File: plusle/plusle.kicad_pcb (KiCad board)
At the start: 2 copper layers, 72.9 x 31 mm, 6 parts, among them J1 Battery, J2 MotorA, J3 MotorB, U1 ESP32-DEVKIT-V1, U2 ROB-14450

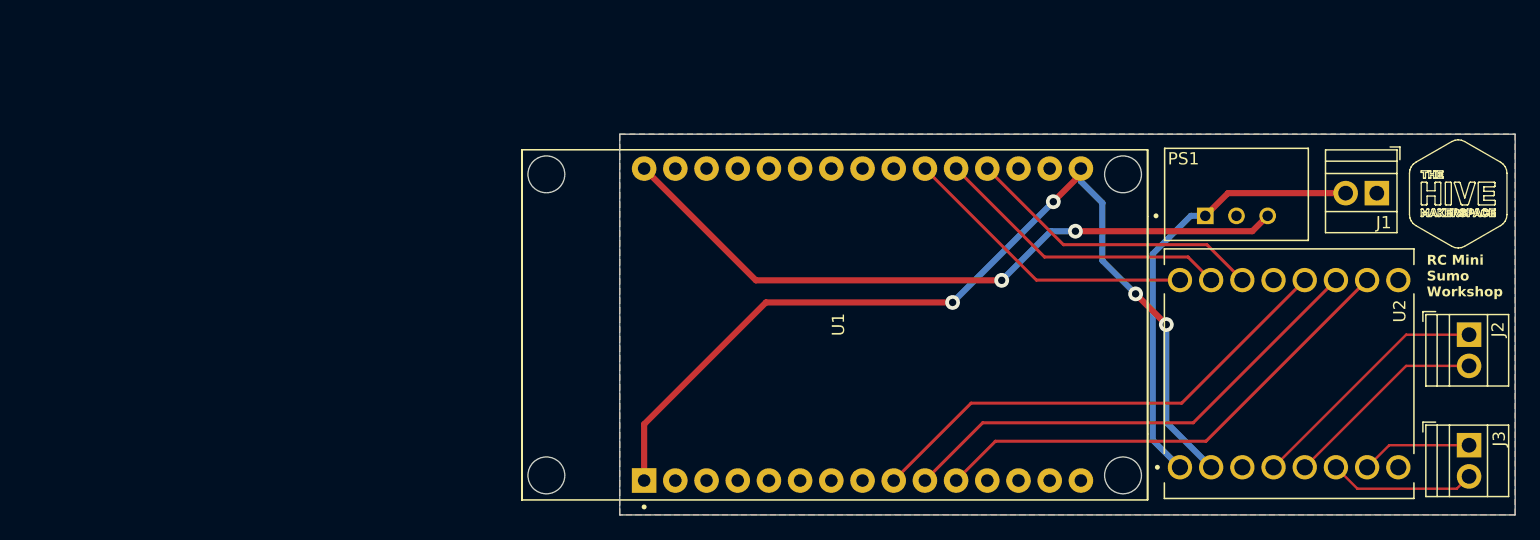
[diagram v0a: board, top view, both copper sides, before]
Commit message: NewIteration
new compact board for personal plusle project, non-hive
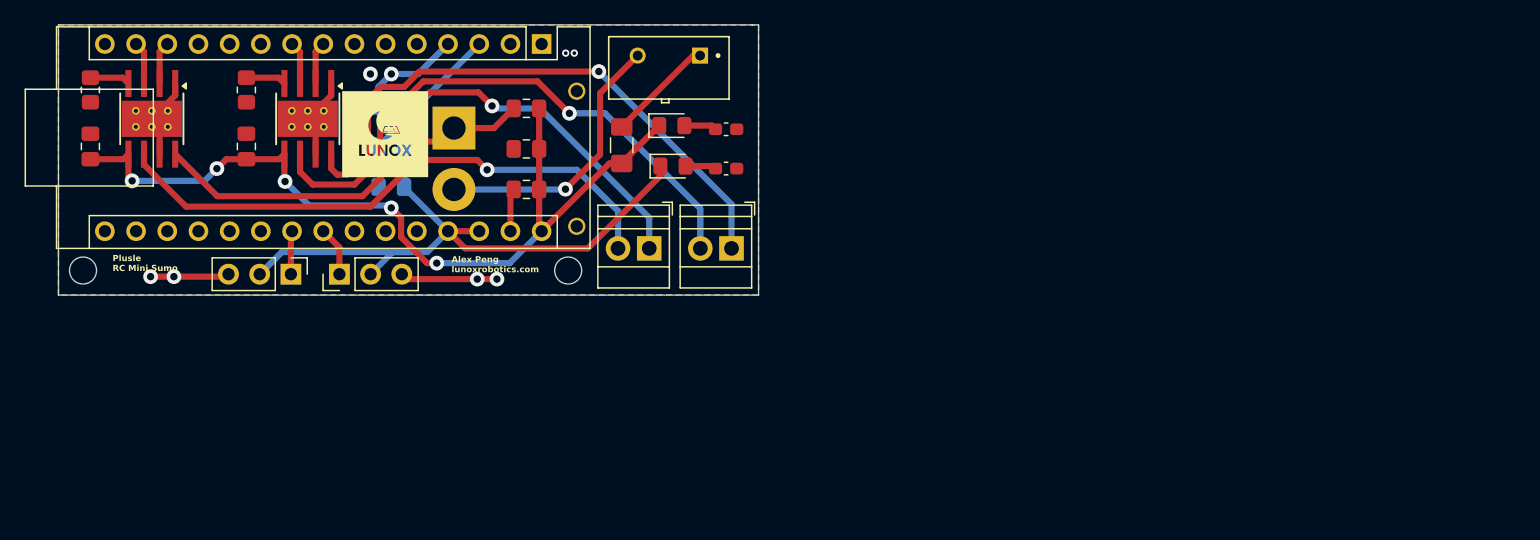
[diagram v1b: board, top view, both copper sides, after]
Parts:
- removed PS1: TSR_1-2450, TSR_1-2433:CONV_TSR_1-2433
- removed U1: ESP32-DEVKIT-V1, Library:MODULE_ESP32_DEVKIT_V1
- removed U2: ROB-14450, Library:MODULE_ROB-14450
- added A1: Arduino_Nano_v3.x, Module:Arduino_Nano, F.Cu at (65.1, 28.2)
- added C1: 0.1uf, Capacitor_SMD:C_0805_2012Metric_Pad1.18x1.45mm_HandSolder, F.Cu at (63.9, 33.4)
- added C2: 0.1uf, Capacitor_SMD:C_0805_2012Metric_Pad1.18x1.45mm_HandSolder, F.Cu at (63.9, 36.7)
- added C3: 0.1uf, Capacitor_SMD:C_0805_2012Metric_Pad1.18x1.45mm_HandSolder, F.Cu at (63.9, 40.0)
- added C4: 0.1uf, Capacitor_SMD:C_0805_2012Metric_Pad1.18x1.45mm_HandSolder, B.Cu at (52.9, 39.8)
- added C5: 0.1uf, Capacitor_SMD:C_0805_2012Metric_Pad1.18x1.45mm_HandSolder, B.Cu at (52.9, 36.5)
- added C6: 0.1uf, Capacitor_SMD:C_0805_2012Metric_Pad1.18x1.45mm_HandSolder, B.Cu at (52.9, 33.2)
- added C7: 0.1uf, Capacitor_SMD:C_0805_2012Metric_Pad1.18x1.45mm_HandSolder, F.Cu at (28.4, 36.5)
- added C8: 0.1uf, Capacitor_SMD:C_0805_2012Metric_Pad1.18x1.45mm_HandSolder, F.Cu at (41.1, 36.5)
- added D1: GREEN, Capacitor_SMD:C_0603_1608Metric_Pad1.08x0.95mm_HandSolder, F.Cu at (80.2, 35.1)
- added D2: GREEN, Capacitor_SMD:C_0603_1608Metric_Pad1.08x0.95mm_HandSolder, F.Cu at (80.2, 38.3)
- added F1: 15A, Fuse:Fuse_1206_3216Metric_Pad1.42x1.75mm_HandSolder, F.Cu at (71.7, 36.4)
- added G***: LOGO, LOGO, F.Cu at (52.4, 35.5)
- added H1: MountingHole, MountingHole:MountingHole_2.2mm_M2_ISO7380, F.Cu at (27.8, 46.6)
- added H2: MountingHole, MountingHole:MountingHole_2.2mm_M2_ISO7380, F.Cu at (67.3, 46.6)
- added J4: Receiver Connection1, Connector_PinHeader_2.54mm:PinHeader_1x03_P2.54mm_Vertical, F.Cu at (44.7, 46.9)
- added J5: Battery, Connector_AMASS:AMASS_XT30PW-M_1x02_P2.50mm_Horizontal, B.Cu at (58.0, 35.0)
- added R1: 15k, Resistor_SMD:R_0805_2012Metric_Pad1.20x1.40mm_HandSolder, F.Cu at (28.4, 31.9)
- added R2: 15k, Resistor_SMD:R_0805_2012Metric_Pad1.20x1.40mm_HandSolder, F.Cu at (41.1, 31.9)
- added R3: 600, Diode_SMD:D_0805_2012Metric_Pad1.15x1.40mm_HandSolder, F.Cu at (75.7, 34.8)
- added R4: 600, Diode_SMD:D_0805_2012Metric_Pad1.15x1.40mm_HandSolder, F.Cu at (75.8, 38.1)
- added SW1: SW_SPST, Button_Switch_THT:SW_AS11CP, F.Cu at (75.5, 30.1)
- added U3: DRV8871DDA, Package_SO:Texas_HTSOP-8-1EP_3.9x4.9mm_P1.27mm_EP2.95x4.9mm_Mask2.4x3.1mm_ThermalVias, F.Cu at (33.4, 34.2)
- added U4: DRV8871DDA, Package_SO:Texas_HTSOP-8-1EP_3.9x4.9mm_P1.27mm_EP2.95x4.9mm_Mask2.4x3.1mm_ThermalVias, F.Cu at (46.1, 34.2)
- J1: value Battery -> Receiver Connection2; footprint TerminalBlock:TerminalBlock_Xinya_XY308-2.54-2P_1x02_P2.54mm_Horizontal -> Connector_PinHeader_2.54mm:PinHeader_1x03_P2.54mm_Vertical
- moved J1 84.7 mm to (48.7, 46.9), turned to 90 degrees
- moved J2 67.1 mm to (73.9, 44.8), turned to 180 degrees
- moved J3 62.2 mm to (80.6, 44.8), turned to 180 degrees
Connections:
- J1 pad 1: GND -> RCSignalB
- J1 pad 2: +12V -> Arduino5V
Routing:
- net +3.3V: track 77.7 -> 0.00 mm, vias 4 -> 0
- net ArduinoVIN: track 0.00 -> 70.0 mm, vias 0 -> 5
- net Arduino5V: track 0.00 -> 67.5 mm
- net +5V: track 56.7 -> 0.00 mm, vias 2 -> 0
- net GND: track 0.00 -> 56.0 mm, vias 0 -> 11
- net PWMB: track 40.2 -> 0.00 mm
- net Net-(J3-Pin_1): track 9.04 -> 48.1 mm, vias 0 -> 1
- net BIn2: track 40.2 -> 3.47 mm
- net BIn1: track 40.2 -> 3.48 mm
- net Net-(J3-Pin_2): track 12.0 -> 48.1 mm, vias 0 -> 1
- net +12V: track 36.0 -> 0.00 mm
- net Net-(J2-Pin_1): track 20.4 -> 52.9 mm, vias 0 -> 1
- net Net-(J2-Pin_2): track 16.8 -> 47.2 mm, vias 0 -> 1
- net PWMA: track 24.5 -> 0.00 mm
- net Net-(J5-Pin_2): track 0.00 -> 22.4 mm, vias 0 -> 1
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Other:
- board size 72.9 x 31 mm -> 57 x 22 mm
- board text added: "Alex Peng lunoxrobotics.com"
- board text added: "Plusle RC Mini Sumo"
- board text removed: "Alex Peng Spring 2025 lunoxrobotics.com"
- board text removed: "RC Mini Sumo Workshop"
